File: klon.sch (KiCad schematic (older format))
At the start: 71 parts, among them SW1 SW_DPDT_x2, U1 TL072, U2 LTC1044, U3 TL072

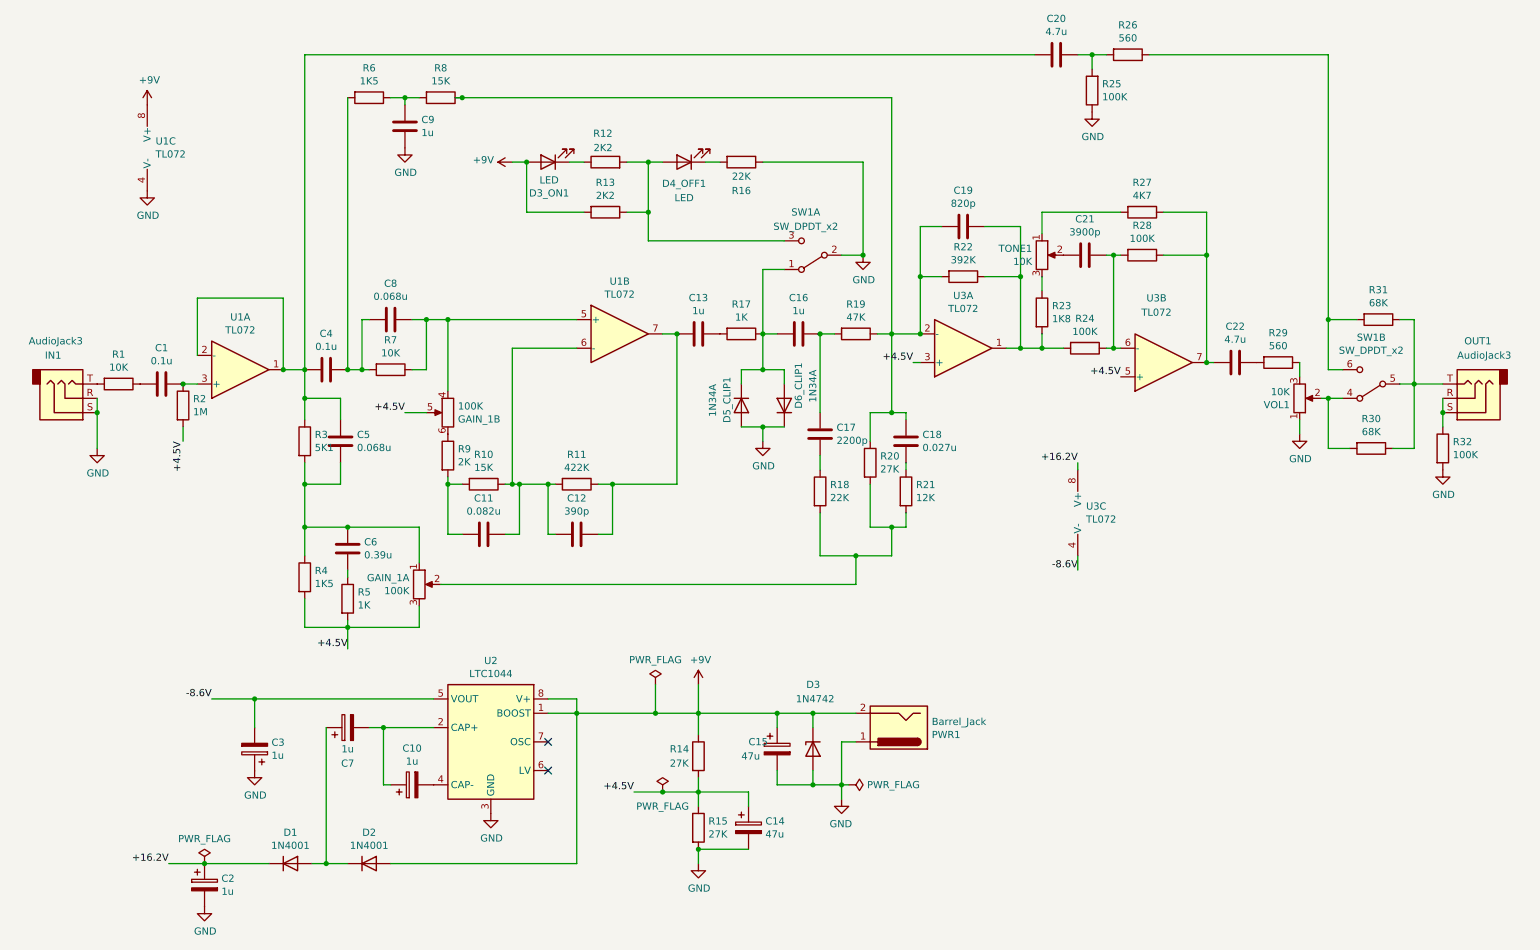
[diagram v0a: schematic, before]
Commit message: update pcb layout
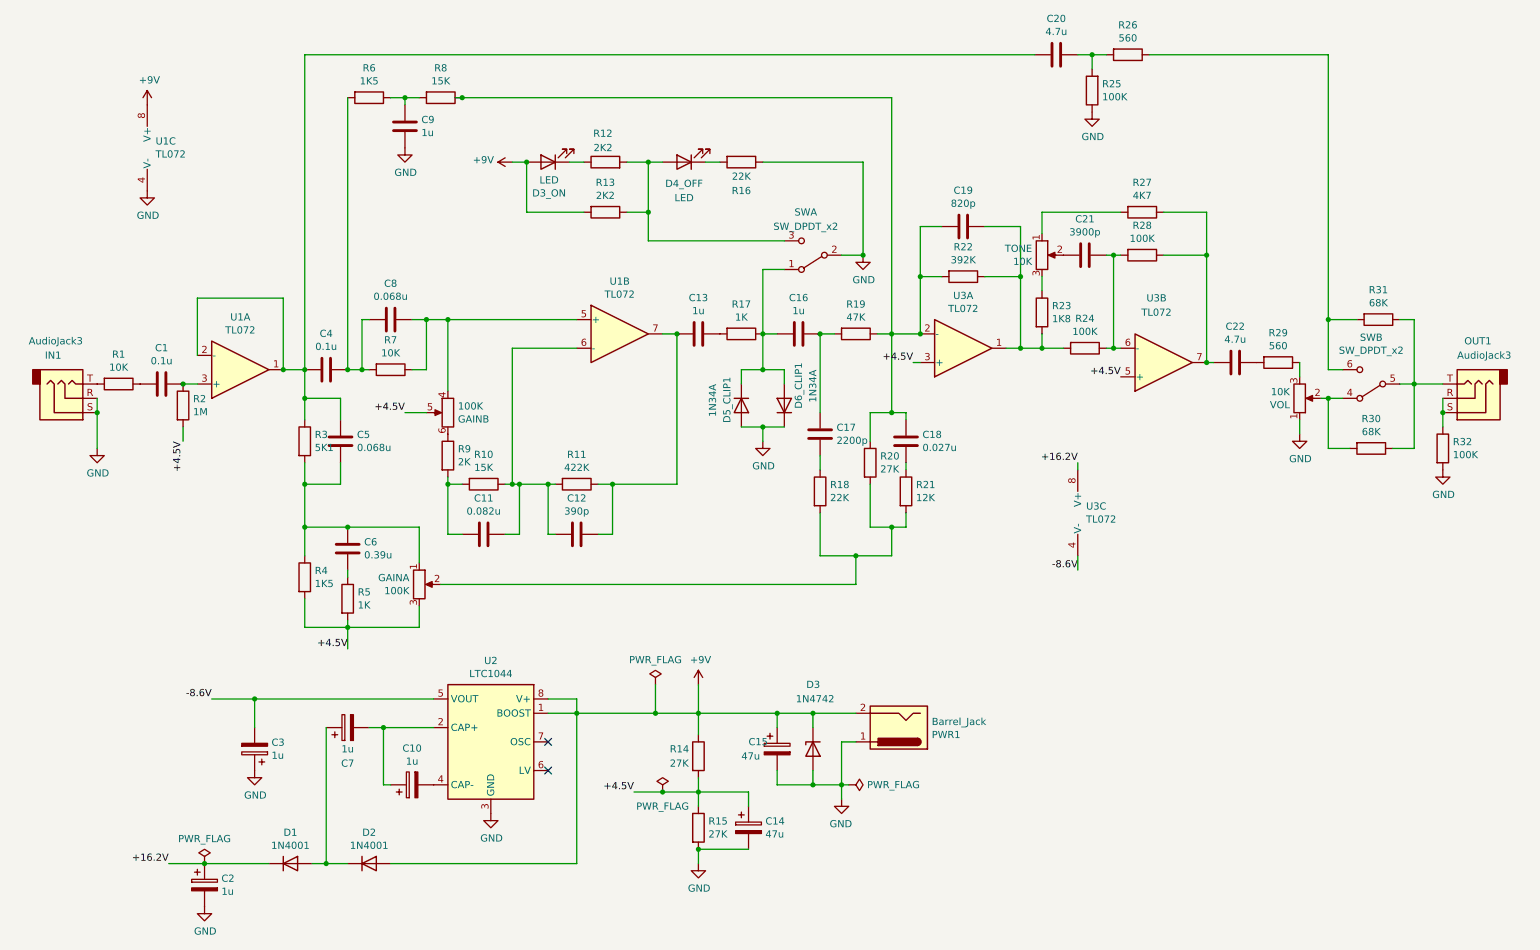
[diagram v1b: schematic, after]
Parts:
- renumbered D3_ON1 to D3_ON, D4_OFF1 to D4_OFF, GAIN_1 to GAIN, SW1 to SW, TONE1 to TONE, VOL1 to VOL
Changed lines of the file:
@@
 	3400 2950 3300 2950
 $Comp
-L klon-rescue:R_POT_Dual_Separate-Device GAIN_1
+L klon-rescue:R_POT_Dual_Separate-Device GAIN
 U 1 1 60CBA9B6
 P 3350 4800
-F 0 "GAIN_1" H 3281 4846 50  0000 R CNN
+F 0 "GAIN" H 3281 4846 50  0000 R CNN
 F 1 "100K" H 3281 4755 50  0000 R CNN
 F 2 "Connector_PinHeader_2.54mm:PinHeader_2x03_P2.54mm_Vertical" H 3350 4800 50  0001 C CNN
@@
 Connection ~ 7550 2650
 $Comp
-L klon-rescue:R_POT-Device TONE1
+L klon-rescue:R_POT-Device TONE
 U 1 1 60D788AD
 P 7700 2500
-F 0 "TONE1" H 7631 2546 50  0000 R CNN
+F 0 "TONE" H 7631 2546 50  0000 R CNN
 F 1 "10K" H 7631 2455 50  0000 R CNN
 F 2 "Connector_PinHeader_2.54mm:PinHeader_1x03_P2.54mm_Vertical" H 7700 2500 50  0001 C CNN
@@
 $EndComp
 $Comp
-L klon-rescue:R_POT-Device VOL1
+L klon-rescue:R_POT-Device VOL
 U 1 1 60DBED2B
 P 9500 3500
-F 0 "VOL1" H 9431 3546 50  0000 R CNN
+F 0 "VOL" H 9431 3546 50  0000 R CNN
 F 1 "10K" H 9431 3455 50  0000 R CNN
 F 2 "Connector_PinHeader_2.54mm:PinHeader_1x03_P2.54mm_Vertical" H 9500 3500 50  0001 C CNN
@@
 	4250 5700 4450 5700
 $Comp
-L Switch:SW_DPDT_x2 SW1
+L Switch:SW_DPDT_x2 SW
 U 2 1 6160A4D6
 P 10000 3400
-F 0 "SW1" H 10000 3075 50  0000 C CNN
+F 0 "SW" H 10000 3075 50  0000 C CNN
 F 1 "SW_DPDT_x2" H 10000 3166 50  0000 C CNN
 F 2 "Connector_PinHeader_2.54mm:PinHeader_2x03_P2.54mm_Vertical" H 10000 3400 50  0001 C CNN
@@
 $EndComp
 $Comp
-L Switch:SW_DPDT_x2 SW1
+L Switch:SW_DPDT_x2 SW
 U 1 1 6160C4D4
 P 6100 2500
-F 0 "SW1" H 6150 2200 50  0000 C CNN
+F 0 "SW" H 6150 2200 50  0000 C CNN
 F 1 "SW_DPDT_x2" H 6150 2300 50  0000 C CNN
 F 2 "Connector_PinHeader_2.54mm:PinHeader_2x03_P2.54mm_Vertical" H 6100 2500 50  0001 C CNN
@@
 	6650 1400 6650 3050
 $Comp
-L Device:LED D3_ON1
+L Device:LED D3_ON
 U 1 1 6161B08C
 P 4250 1850
-F 0 "D3_ON1" H 4243 2067 50  0000 C CNN
+F 0 "D3_ON" H 4243 2067 50  0000 C CNN
 F 1 "LED" H 4243 1976 50  0000 C CNN
 F 2 "LED_THT:LED_D3.0mm_Clear" H 4250 1850 50  0001 C CNN
@@
 Connection ~ 4950 2200
 $Comp
-L klon-rescue:R_POT_Dual_Separate-Device GAIN_1
+L klon-rescue:R_POT_Dual_Separate-Device GAIN
 U 2 1 60CB9AA2
 P 3550 3600
-F 0 "GAIN_1" H 3480 3554 50  0000 R CNN
+F 0 "GAIN" H 3480 3554 50  0000 R CNN
 F 1 "100K" H 3480 3645 50  0000 R CNN
 F 2 "Connector_PinHeader_2.54mm:PinHeader_2x03_P2.54mm_Vertical" H 3550 3600 50  0001 C CNN
@@
 	6150 4000 6150 3900
 $Comp
-L Device:LED D4_OFF1
+L Device:LED D4_OFF
 U 1 1 61235DB3
 P 5200 1850
-F 0 "D4_OFF1" H 5200 2000 50  0000 C CNN
+F 0 "D4_OFF" H 5200 2000 50  0000 C CNN
 F 1 "LED" H 5200 2100 50  0000 C CNN
 F 2 "LED_THT:LED_D3.0mm_Clear" H 5200 1850 50  0001 C CNN
